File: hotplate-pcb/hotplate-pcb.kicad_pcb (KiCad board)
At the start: 2 copper layers, 2 parts

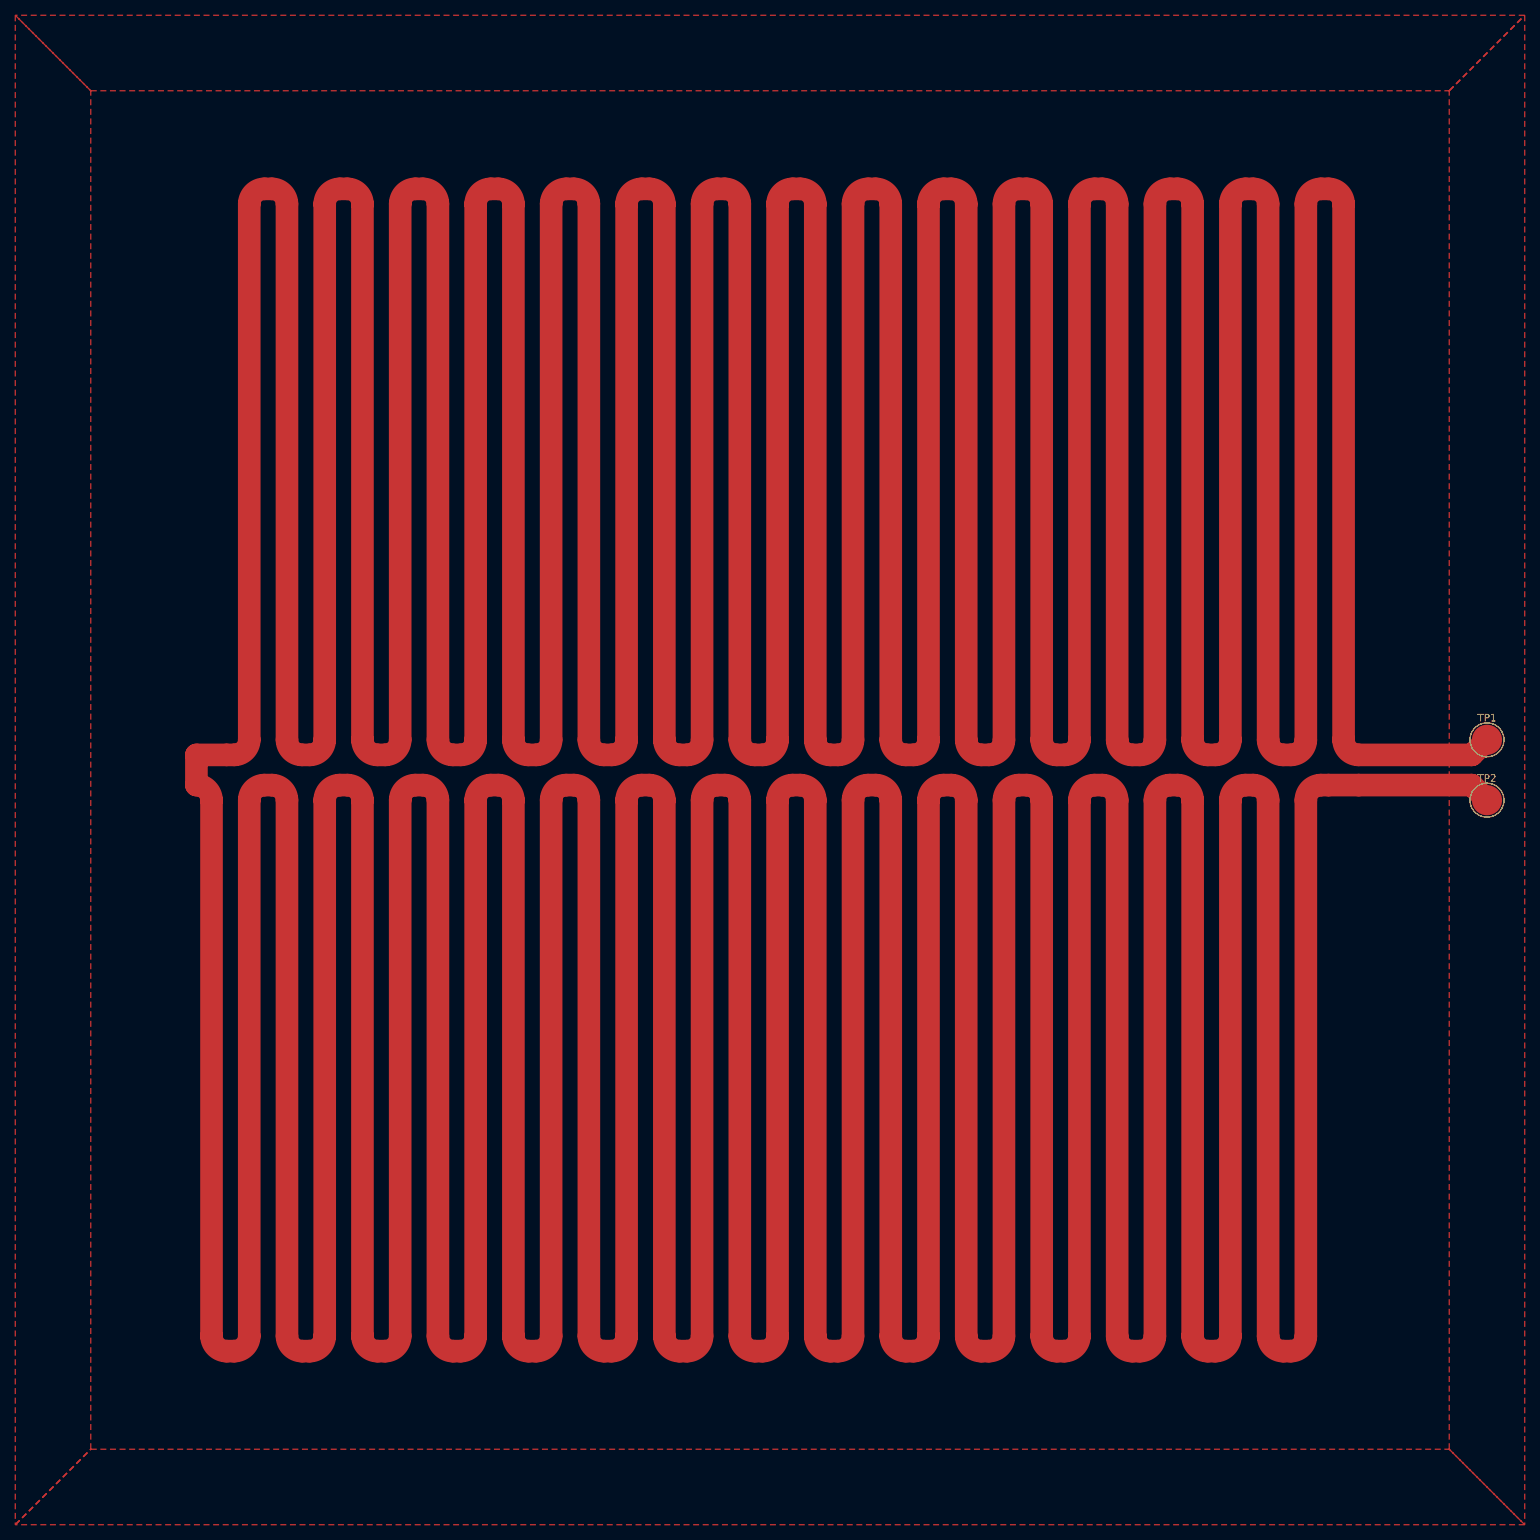
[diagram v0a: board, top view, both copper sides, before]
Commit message: 2025-06-09
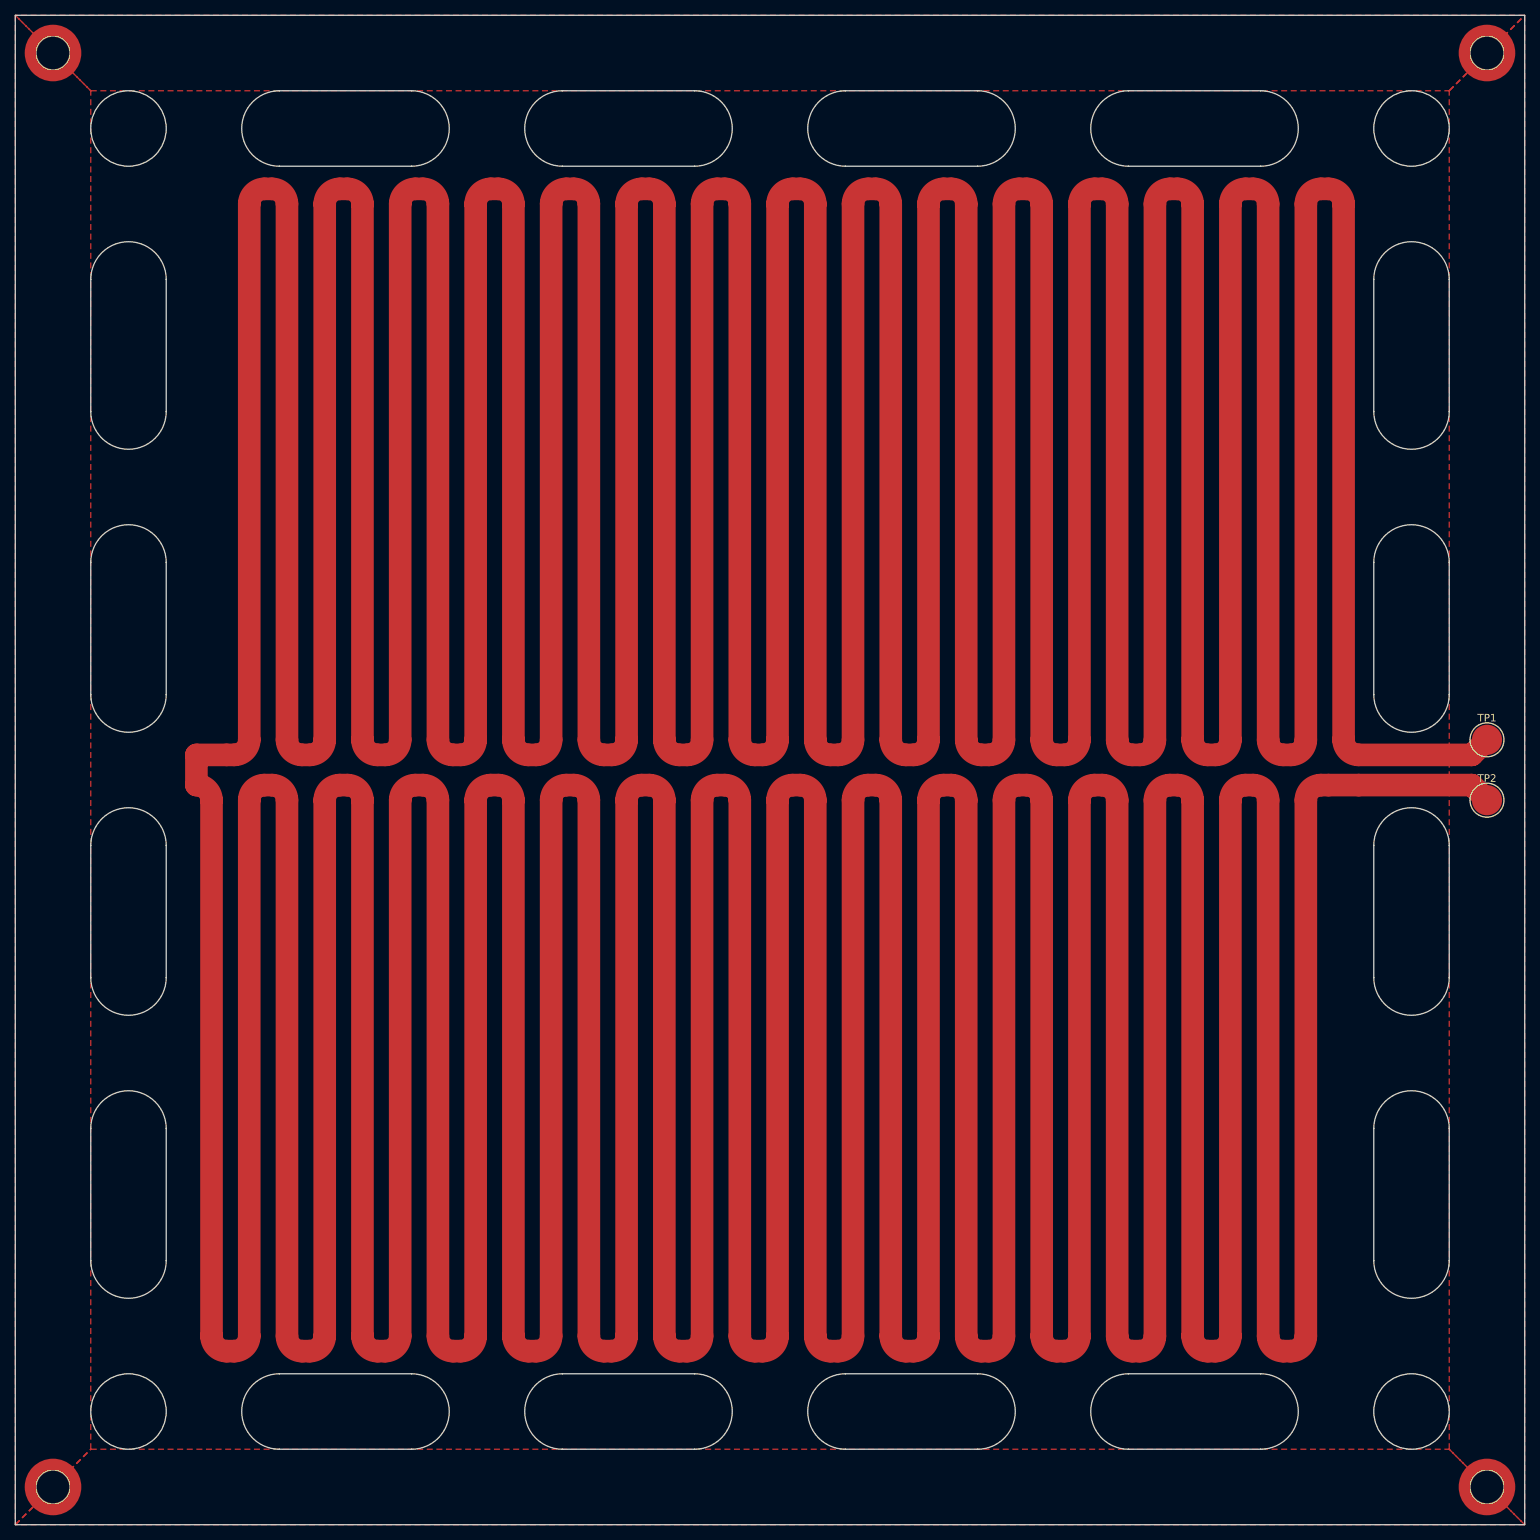
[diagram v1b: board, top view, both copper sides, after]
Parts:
- added REF**: MountingHole_4.3mm_M4_DIN965_Pad_TopOnly, MountingHole:MountingHole_4.3mm_M4_DIN965_Pad_TopOnly, F.Cu at (295.0, 235.0)
- added REF**: MountingHole_4.3mm_M4_DIN965_Pad_TopOnly, MountingHole:MountingHole_4.3mm_M4_DIN965_Pad_TopOnly, F.Cu at (105.0, 45.0)
- added REF**: MountingHole_4.3mm_M4_DIN965_Pad_TopOnly, MountingHole:MountingHole_4.3mm_M4_DIN965_Pad_TopOnly, F.Cu at (295.0, 45.0)
- added REF**: MountingHole_4.3mm_M4_DIN965_Pad_TopOnly, MountingHole:MountingHole_4.3mm_M4_DIN965_Pad_TopOnly, F.Cu at (105.0, 235.0)
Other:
- board outline added: 200 x 200 mm
